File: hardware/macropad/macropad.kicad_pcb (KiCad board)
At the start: 2 copper layers, 162.9 x 95.3 mm, 93 parts, among them J1 SWD, J10 Conn_01x02, J2 USB_C_Receptacle_USB2.0_16P, J3 Conn_01x02, J4 display(4x1), J5 Conn_01x04_Pin, J6 Conn_01x03_Socket, J8 Conn_01x02, J9 USB_A, Q1 Q_PMOS, Q2 FS8205A, SW1 SW_Push, SW10 SW_SPDT, SW12 RotaryEncoder_Switch, SW13 RotaryEncoder_Switch, SW2 SW_Push, SW3 SW_Push, SW4 SW_Push, SW5 SW_Push, SW6 SW_Push, SW7 SW_Push, SW8 SW_Push, SW9 SW_Push, U1 LP2992IM5-3.3/NOPB, U2 STM32F103C8Tx, U3 NRF24L01_Breakout, U4 STM32F103C8Tx, U5 NRF24L01_Breakout, U6 TP4056-42-ESOP8, U7 DW01A, U9 LP2992IM5-3.3/NOPB, Y1 8Mhz C_L=12pF, Y2 8Mhz

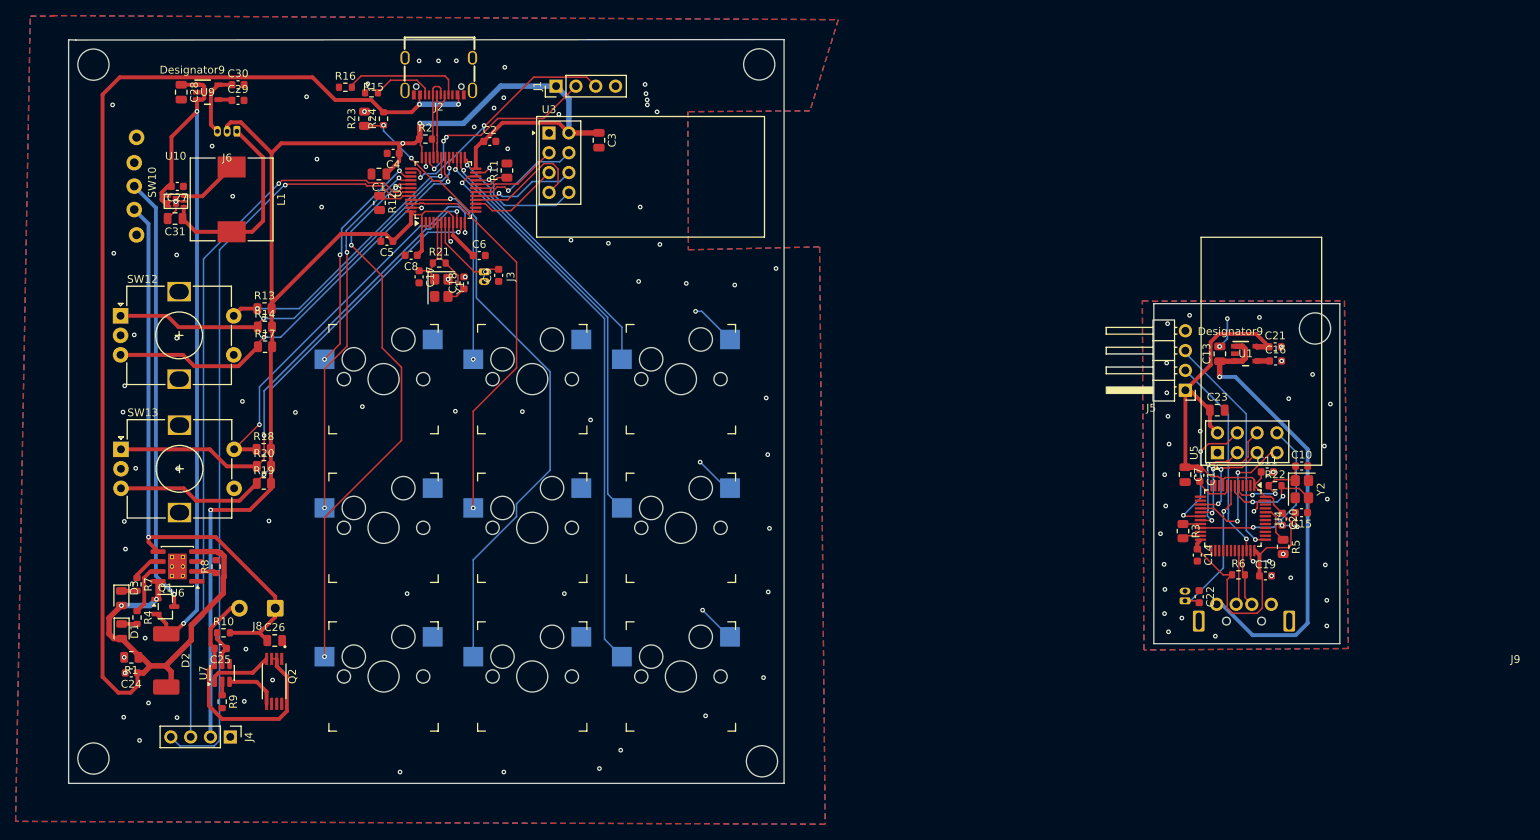
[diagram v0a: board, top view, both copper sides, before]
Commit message: stitching done
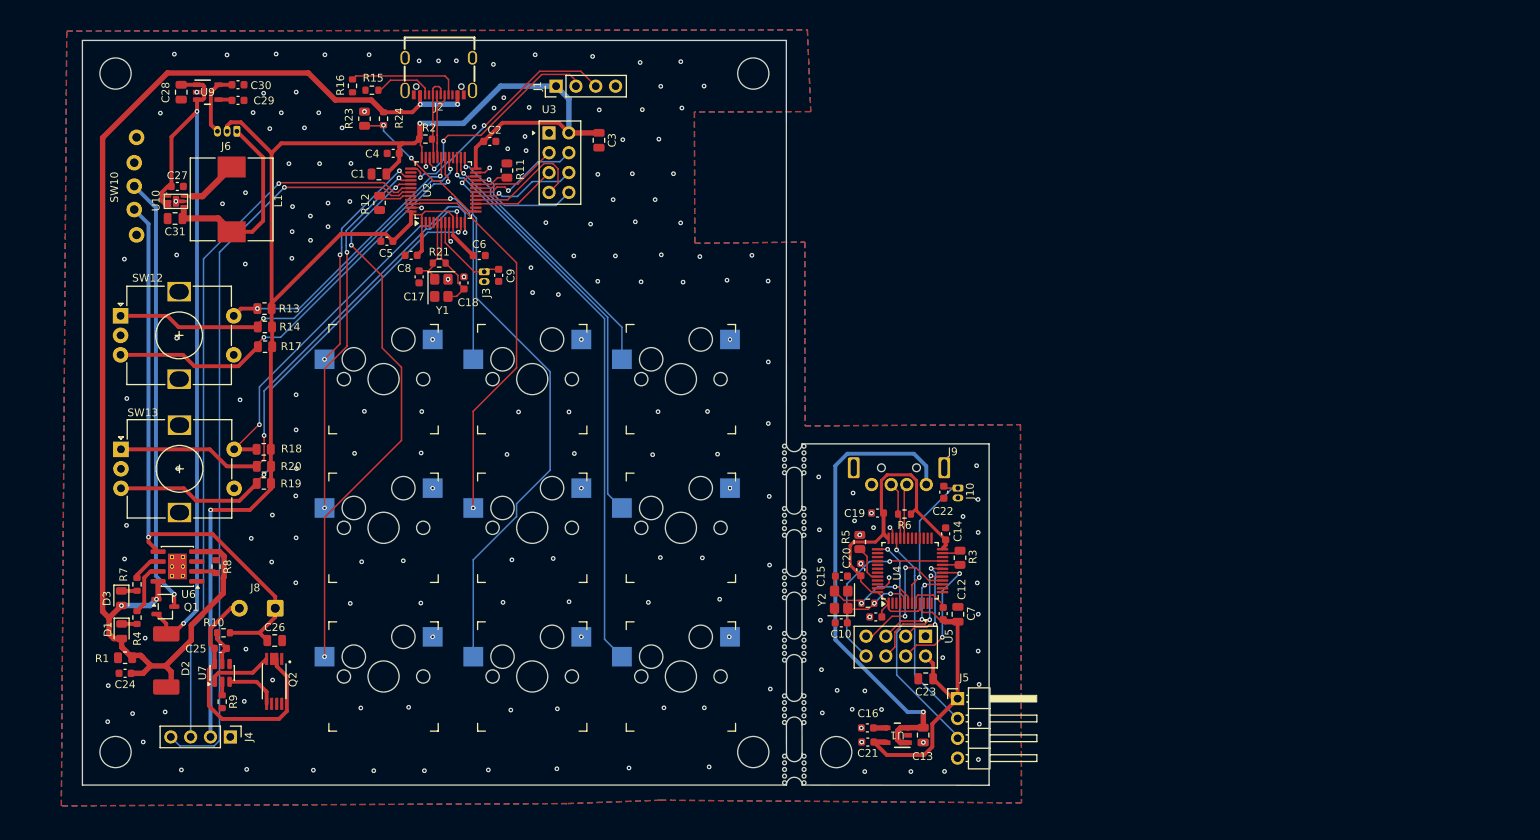
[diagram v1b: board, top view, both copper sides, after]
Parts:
- added REF**: MouseBite-Slot_2.0x2.0mm_inset_D0.5mm_P0.85mm_5h, Panelization:MouseBite-Slot_2.0x2.0mm_inset_D0.5mm_P0.85mm_5h, F.Cu at (140.6, 135.5)
- added REF**: MouseBite-Slot_2.0x2.0mm_inset_D0.5mm_P0.85mm_5h, Panelization:MouseBite-Slot_2.0x2.0mm_inset_D0.5mm_P0.85mm_5h, F.Cu at (142.6, 95.8)
- added REF**: MouseBite-Slot_2.0x2.0mm_inset_D0.5mm_P0.85mm_5h, Panelization:MouseBite-Slot_2.0x2.0mm_inset_D0.5mm_P0.85mm_5h, F.Cu at (142.6, 127.8)
- added REF**: MouseBite-Slot_2.0x2.0mm_inset_D0.5mm_P0.85mm_5h, Panelization:MouseBite-Slot_2.0x2.0mm_inset_D0.5mm_P0.85mm_5h, F.Cu at (142.6, 111.8)
- added REF**: MouseBite-Slot_2.0x2.0mm_inset_D0.5mm_P0.85mm_5h, Panelization:MouseBite-Slot_2.0x2.0mm_inset_D0.5mm_P0.85mm_5h, F.Cu at (142.6, 103.8)
- added REF**: MouseBite-Slot_2.0x2.0mm_inset_D0.5mm_P0.85mm_5h, Panelization:MouseBite-Slot_2.0x2.0mm_inset_D0.5mm_P0.85mm_5h, F.Cu at (142.6, 119.8)
- moved C21 72.7 mm to (151.0, 132.0), turned to 180 degrees
- moved C16 70.3 mm to (151.0, 130.1), turned to 180 degrees
- moved U1 66.2 mm to (154.8, 131.1), turned to 180 degrees
- moved C10 62.3 mm to (147.6, 116.7), turned to 180 degrees
- moved C13 61.9 mm to (158.1, 131.1), turned to -90 degrees
- moved Y2 60.7 mm to (147.6, 113.7), turned to 90 degrees
- moved C15 59.5 mm to (147.6, 110.7), turned to 0 degrees
- moved C20 54.4 mm to (150.1, 109.9), turned to 90 degrees
- moved R22 54.3 mm to (151.0, 114.2), turned to 180 degrees
- moved R5 54.3 mm to (150.0, 106.3), turned to 90 degrees
- moved C11 53.5 mm to (152.0, 115.9), turned to 180 degrees
- moved C23 50.8 mm to (158.4, 123.8), turned to 180 degrees
- moved C19 50.4 mm to (152.3, 102.6), turned to 180 degrees
- moved J5 49.1 mm to (162.5, 126.4), turned to 0 degrees
- moved J9 48.4 mm to (155.0, 96.8), turned to 180 degrees
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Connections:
- C10 pad 2: GND_DGL -> GND
- C11 pad 2: GND_DGL -> GND
- C12 pad 2: GND_DGL -> GND
- C13 pad 2: GND_DGL -> GND
- C14 pad 2: GND_DGL -> GND
- C15 pad 2: GND_DGL -> GND
- C16 pad 2: GND_DGL -> GND
- C19 pad 2: GND_DGL -> GND
- C20 pad 2: GND_DGL -> GND
- C21 pad 2: GND_DGL -> GND
- C22 pad 1: GND_DGL -> GND
- C23 pad 2: GND_DGL -> GND
- C7 pad 2: GND_DGL -> GND
- J10 pad 2: GND_DGL -> GND
- J5 pad 4: GND_DGL -> GND
- J9 pad 4: GND_DGL -> GND
- J9 pad 5: GND_DGL -> GND
- R3 pad 2: GND_DGL -> GND
- R5 pad 2: GND_DGL -> GND
- U1 pad 2: GND_DGL -> GND
- U4 pad 23: GND_DGL -> GND
- U4 pad 35: GND_DGL -> GND
- U4 pad 47: GND_DGL -> GND
- U4 pad 8: GND_DGL -> GND
- U5 pad 1: GND_DGL -> GND
- Y2 pad 2: GND_DGL -> GND
- Y2 pad 4: GND_DGL -> GND
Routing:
- net GND_DGL: track 22.1 -> 0.00 mm, vias 38 -> 0
- net VBUS: track 180.5 -> 161.8 mm
- net GND: track 27.7 -> 20.3 mm, vias 80 -> 197
- net /dongle/HSE_IN_DGL: track 12.8 -> 11.0 mm
- net /SWDIO: track 25.7 -> 27.4 mm, vias 3 -> 2
- net VBUS_DGL: track 59.4 -> 60.8 mm
- net /Power/Vout_buck: track 26.1 -> 24.7 mm
- net /dongle/HSE_OUT_DGL: track 15.3 -> 14.3 mm
- net /PA5: track 11.8 -> 11.0 mm
- net Net-(J2-CC1): track 15.3 -> 14.7 mm
- net /Power/B-: track 34.2 -> 33.6 mm
- net /SWCLK: track 30.5 -> 31.1 mm
- net /SDAPB7: track 98.7 -> 98.1 mm
- net /K4: vias 2 -> 1
- net +3.3V: vias 3 -> 2
- removed copper zone on B.Cu, net GND_DGL
- removed copper zone on F.Cu, net GND_DGL
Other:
- board size 162.9 x 95.3 mm -> 116.2 x 95.4 mm

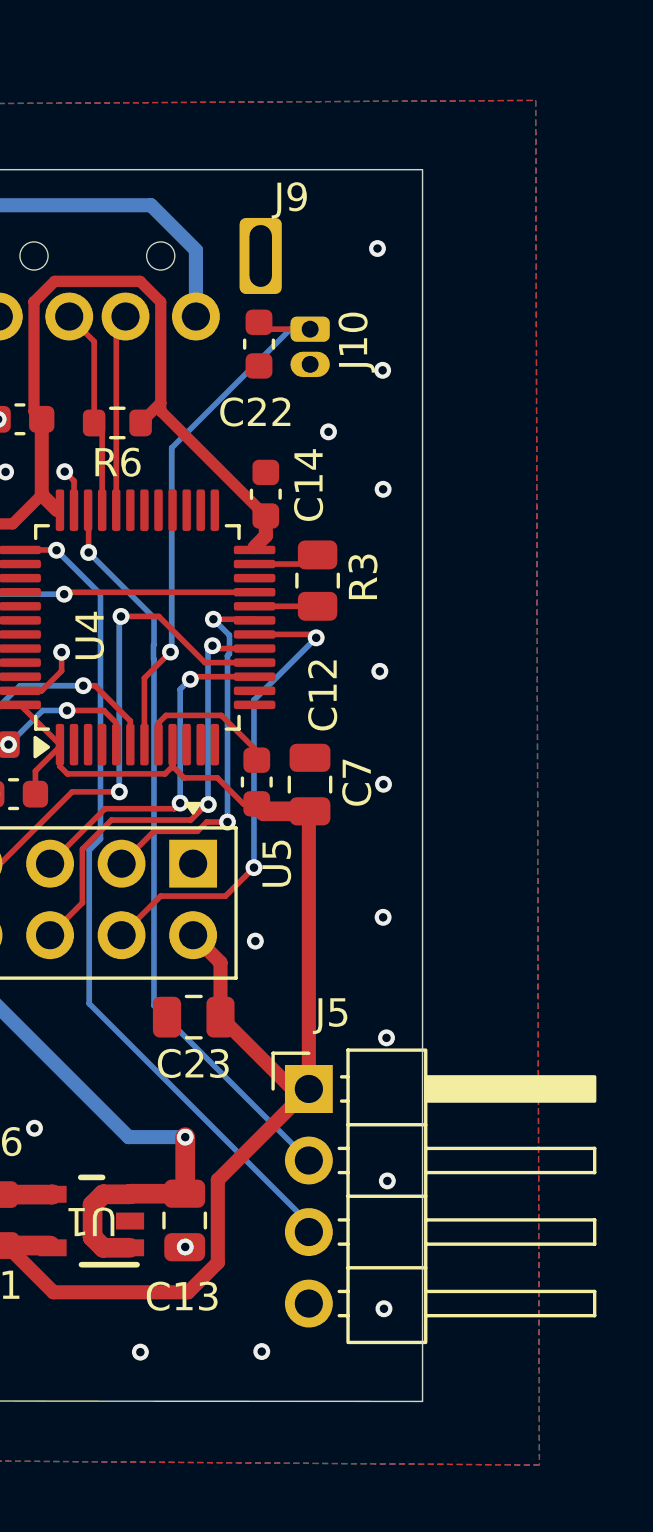
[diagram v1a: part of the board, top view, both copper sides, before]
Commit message: fab outputs
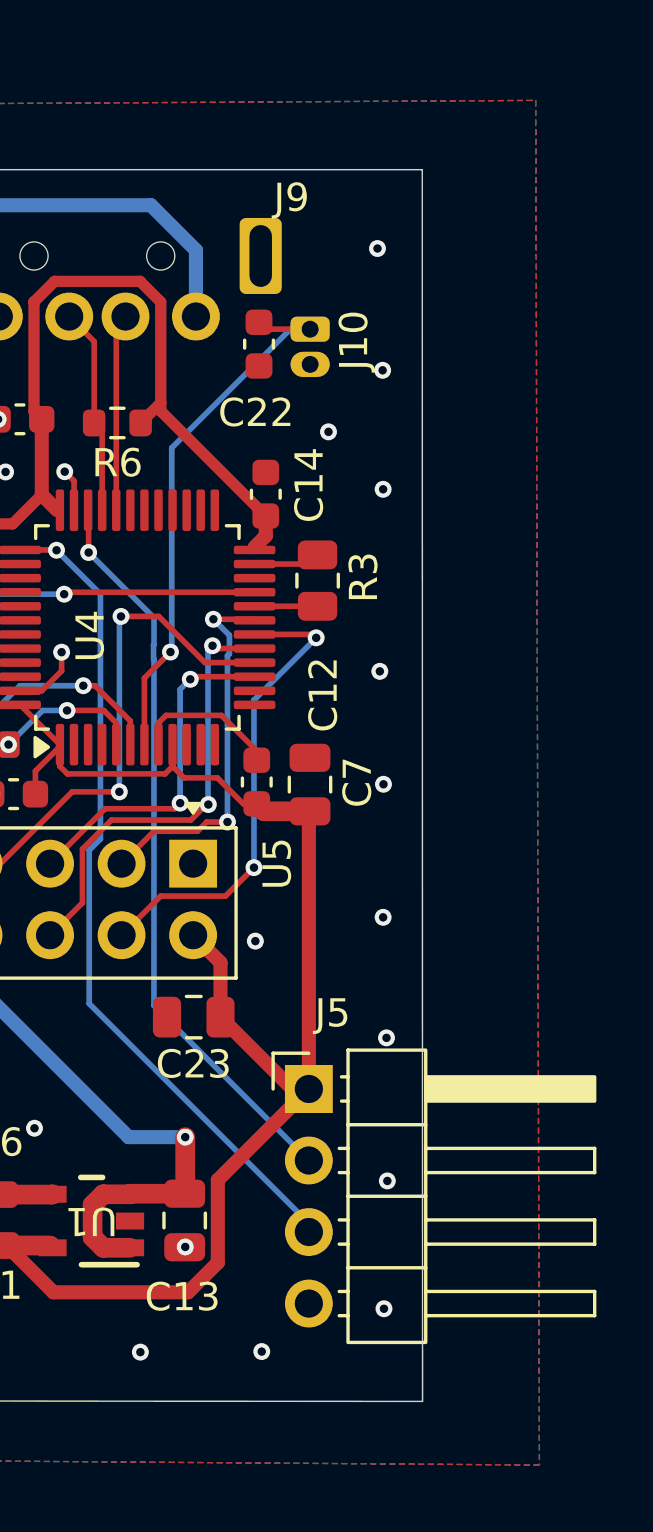
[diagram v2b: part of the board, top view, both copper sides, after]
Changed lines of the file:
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@@
 			(outputformat 1)
 			(mirror no)
-			(drillshape 1)
+			(drillshape 0)
 			(scaleselection 1)
-			(outputdirectory "")
+			(outputdirectory "./")
 		)
 	)
@@
 		(tags "connector Hirose DF13 vertical")
 		(property "Reference" "J10"
-			(at 0.395 -1.562024 -90)
+			(at 0.395 -1.562024 270)
 			(layer "F.SilkS")
 			(effects
@@
 	)
 	(gr_line
-		(start 166.55 137.49)
-		(end 166.55 93.75)
+		(start 166.54 93.75)
+		(end 166.55 137.49)
 		(stroke
 			(width 0.05)

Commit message: proper fab outs
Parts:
- C24, C25: value 0.1u -> 100n
- R6: value 1.5K -> 1.5k
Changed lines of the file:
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@@
 		(sheetname "/Power/")
 		(sheetfile "macropad_power.kicad_sch")
-		(attr through_hole)
+		(attr through_hole dnp)
 		(pad "1" thru_hole roundrect
 			(at 0 0 180)
@@
 		(sheetname "/")
 		(sheetfile "macropad.kicad_sch")
-		(attr smd)
+		(attr smd dnp)
 		(fp_line
 			(start -7 -6)
@@
 		(sheetname "/")
 		(sheetfile "macropad.kicad_sch")
-		(attr smd)
+		(attr smd dnp)
 		(fp_line
 			(start -7 -6)
@@
 		(sheetname "/")
 		(sheetfile "macropad.kicad_sch")
-		(attr smd)
+		(attr smd dnp)
 		(fp_line
 			(start -7 -6)
@@
 		(sheetname "/")
 		(sheetfile "macropad.kicad_sch")
-		(attr smd)
+		(attr smd dnp)
 		(fp_line
 			(start -7 -6)
@@
 		(sheetname "/dongle/")
 		(sheetfile "dongle.kicad_sch")
-		(attr smd)
+		(attr smd dnp)
 		(fp_rect
 			(start -5.8 3.125)
@@
 		(sheetname "/")
 		(sheetfile "macropad.kicad_sch")
-		(attr through_hole)
+		(attr through_hole dnp)
 		(fp_line
 			(start -0.3 -1.6)
@@
 		(sheetname "/")
 		(sheetfile "macropad.kicad_sch")
-		(attr smd)
+		(attr smd dnp)
 		(fp_line
 			(start -7 -6)
@@
 		(sheetname "/Power/")
 		(sheetfile "macropad_power.kicad_sch")
-		(attr smd)
+		(attr smd dnp)
 		(fp_rect
 			(start -2 -11.5)
@@
 		(sheetname "/Power/")
 		(sheetfile "macropad_power.kicad_sch")
-		(attr exclude_from_pos_files)
+		(attr exclude_from_pos_files dnp)
 		(fp_rect
 			(start 2.8 -1.58)
@@
 		(sheetname "/")
 		(sheetfile "macropad.kicad_sch")
-		(attr through_hole)
+		(attr through_hole dnp)
 		(pad "1" thru_hole roundrect
 			(at 0 0 270)
@@
 		(sheetname "/")
 		(sheetfile "macropad.kicad_sch")
-		(attr through_hole)
+		(attr through_hole dnp)
 		(fp_line
 			(start -0.3 -1.6)
@@
 		(sheetname "/")
 		(sheetfile "macropad.kicad_sch")
-		(attr smd)
+		(attr smd dnp)
 		(fp_line
 			(start -7 -6)
@@
 			)
 		)
-		(property "Value" "0.1u"
+		(property "Value" "100n"
 			(at 0 1.43 0)
 			(layer "F.Fab")
@@
 		(sheetname "/")
 		(sheetfile "macropad.kicad_sch")
-		(attr smd)
+		(attr smd dnp)
 		(fp_line
 			(start -7 -6)
@@
 		(sheetname "/")
 		(sheetfile "macropad.kicad_sch")
-		(attr smd)
+		(attr smd dnp)
 		(fp_line
 			(start -7 -6)
@@
 		(sheetname "/")
 		(sheetfile "macropad.kicad_sch")
-		(attr through_hole)
+		(attr through_hole dnp)
 		(fp_line
 			(start -1.38 -1.38)
@@
 			)
 		)
-		(property "Value" "0.1u"
+		(property "Value" "100n"
 			(at 0 1.43 0)
 			(layer "F.Fab")
@@
 		(sheetname "/")
 		(sheetfile "macropad.kicad_sch")
-		(attr through_hole)
+		(attr through_hole dnp)
 		(fp_line
 			(start -1.38 9)
@@
 		(sheetname "/dongle/")
 		(sheetfile "dongle.kicad_sch")
-		(attr through_hole)
+		(attr through_hole dnp)
 		(fp_line
 			(start -1.27 -1.27)
@@
 			)
 		)
-		(property "Value" "1.5K"
+		(property "Value" "1.5k"
 			(at 0 1.43 0)
 			(layer "F.Fab")
@@
 		(sheetname "/")
 		(sheetfile "macropad.kicad_sch")
-		(attr smd)
+		(attr smd dnp)
 		(fp_line
 			(start -7 -6)
@@
 		(sheetname "/dongle/")
 		(sheetfile "dongle.kicad_sch")
-		(attr through_hole)
+		(attr through_hole dnp)
 		(fp_text user "${REFERENCE}"
 			(at 0.62 1.5 90)
